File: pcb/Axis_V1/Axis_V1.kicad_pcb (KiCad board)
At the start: 2 copper layers, 63.5 x 101.6 mm, 40 parts, among them J1 TRANSDUCER, J10 Conn_01x03, J11 3WAY_L, J12 Conn_01x03, J2 Screw_Terminal_01x03, J3 BREW_SW, J4 STEAM_SW, J5 AC_L, J6 AC_N, J7 BOILER_SSR, J8 Screw_Terminal_01x02, J9 PUMP_L, Q1 BC847, Q2 BT136S-600, Q3 BT136S-600, U1 Pico, U2 ADS1115IDGS, U3 MAX31855KASA

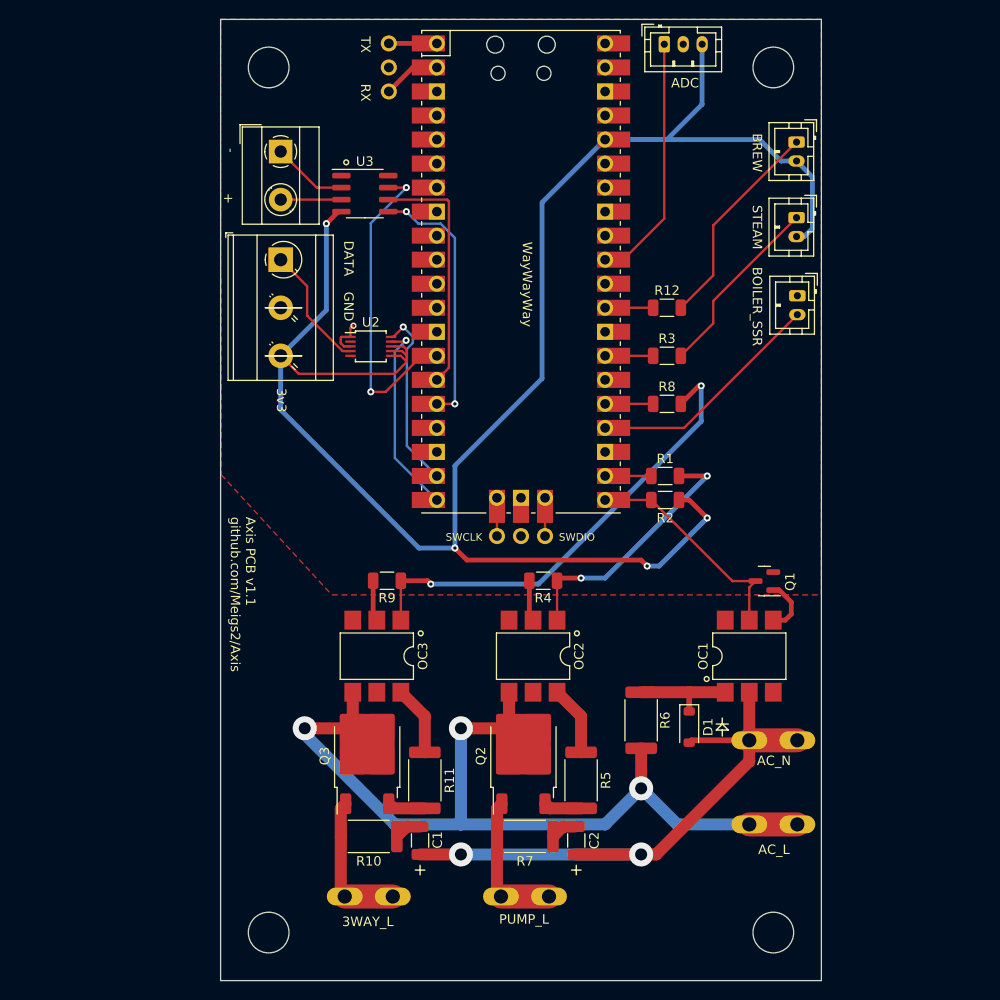
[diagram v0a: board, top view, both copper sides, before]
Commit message: Almost messed it up.
Moved things around and make sure the rust code and schematics match up.
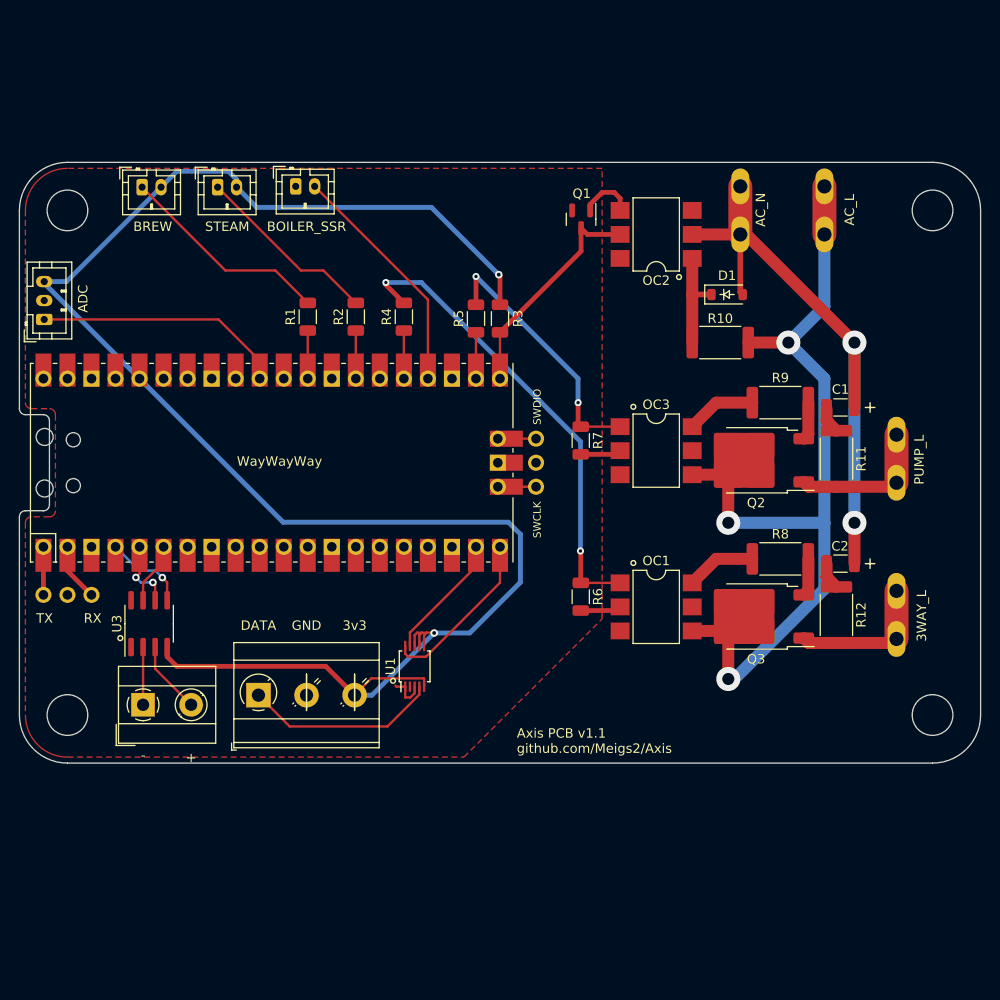
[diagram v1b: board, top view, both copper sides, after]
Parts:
- D1: value RFN1LAM6STR -> HS1MFL
- Q2, Q3: value BT136S-600 -> ACST410-8BTR
- R10: renamed from R6; value 20k -> 56k
- moved H3 78.2 mm to (198.1, 68.6), turned to 0 degrees
- moved H4 76.1 mm to (106.7, 68.6), turned to 0 degrees
- moved H2 73.8 mm to (198.1, 121.9), turned to 0 degrees
- moved J10 71.7 mm to (104.2, 80.1), turned to 90 degrees
- moved H1 71.7 mm to (106.7, 121.9), turned to 0 degrees
- moved J6 69.3 mm to (114.6, 66.1), turned to 0 degrees
- moved J3 65.3 mm to (106.7, 109.2), turned to 180 degrees
- moved J11 65.1 mm to (186.7, 68.6), turned to 90 degrees
- moved J9 63.2 mm to (194.3, 111.3), turned to 90 degrees
- moved J7 61.3 mm to (122.6, 66.1), turned to 0 degrees
- moved J8 60.7 mm to (194.3, 94.8), turned to 90 degrees
- moved J4 60.3 mm to (114.7, 120.8), turned to 0 degrees
- moved J12 56.1 mm to (177.8, 68.6), turned to 90 degrees
- moved R12 54.7 mm to (188.0, 111.3), turned to -90 degrees
- moved J2 54.3 mm to (130.8, 66.0), turned to 0 degrees
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- renumbered C2 to C1, C1 to C2, J2 to J10, J5 to J11, J6 to J12, J7 to J2, J10 to J3, J8 to J4, J12 to J5, J3 to J6, J4 to J7, J9 to J8, J11 to J9, OC3 to OC1, OC1 to OC2, OC2 to OC3, R12 to R1, R7 to R11, R10 to R12, R3 to R2, R2 to R3, R8 to R4, R1 to R5, R9 to R6, R4 to R7, R11 to R8, R5 to R9, U2 to U1, U1 to U2
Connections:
- U1 pad 10: /ADS_SDA -> /ADS_SCL
- U1 pad 9: /ADS_SCL -> /ADS_SDA
- U2 pad 14: /MAX_SO -> unconnected-(U2-GPIO10-Pad14)
- U2 pad 15: /MAX_CS -> unconnected-(U2-GPIO11-Pad15)
- U2 pad 16: /MAX_SCL -> unconnected-(U2-GPIO12-Pad16)
- U2 pad 4: unconnected-(U1-GPIO2-Pad4) -> /MAX_SCL
- U2 pad 5: unconnected-(U1-GPIO3-Pad5) -> /MAX_CS
- U2 pad 6: unconnected-(U1-GPIO4-Pad6) -> /MAX_MISO
- U3 pad 7: /MAX_SO -> /MAX_MISO
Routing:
- net /MAX_SO: track 33.6 -> 0.00 mm, vias 2 -> 0
- net /MAX_SCL: track 27.6 -> 8.91 mm, vias 2 -> 1
- net /MAX_CS: track 25.9 -> 7.40 mm, vias 0 -> 2
- net +3.3V: track 201.3 -> 188.0 mm, vias 4 -> 2
- net /PRES_SENS: track 13.2 -> 20.6 mm
- net /MAX_MISO: track 0.00 -> 6.55 mm
- net /ADS_SDA: track 19.5 -> 13.4 mm, vias 1 -> 0
- net /ADS_SCL: track 20.9 -> 18.0 mm, vias 1 -> 0
- net /NEG_THCPL: track 7.99 -> 6.10 mm
- net /POS_THCPL: track 6.41 -> 7.67 mm
- net /AC_N: track 64.6 -> 63.6 mm
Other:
- board size 63.5 x 101.6 mm -> 101.6 x 63.5 mm
